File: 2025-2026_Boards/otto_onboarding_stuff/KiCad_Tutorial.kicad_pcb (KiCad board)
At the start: 2 copper layers, 28 parts, among them J1 USB_B_Micro, J2 Conn_01x04_Pin, J3 Conn_01x04_Pin, J4 Conn_01x04_Pin, SW1 SW_SPDT, U1 STM32F103C8T6, U3 AMS1117-3.3, Y1 16MHz

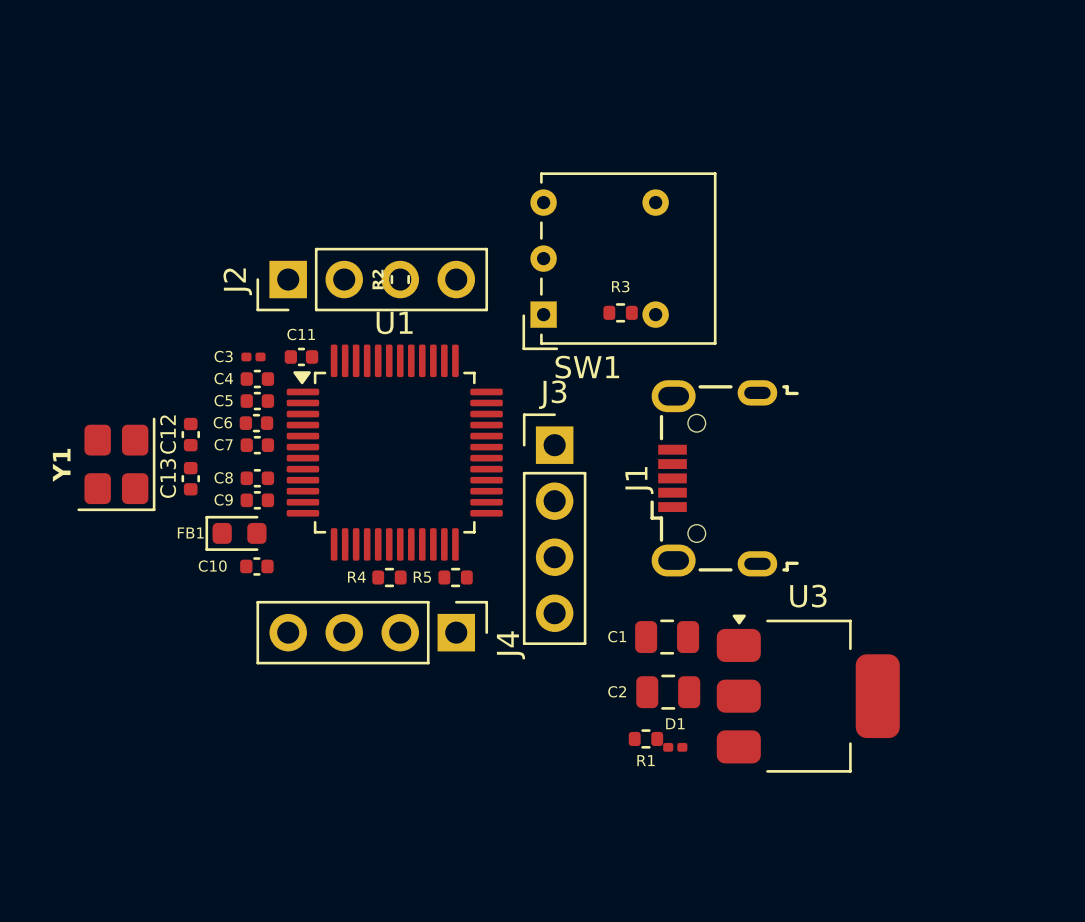
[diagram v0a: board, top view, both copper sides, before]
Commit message: Worked on wiring.
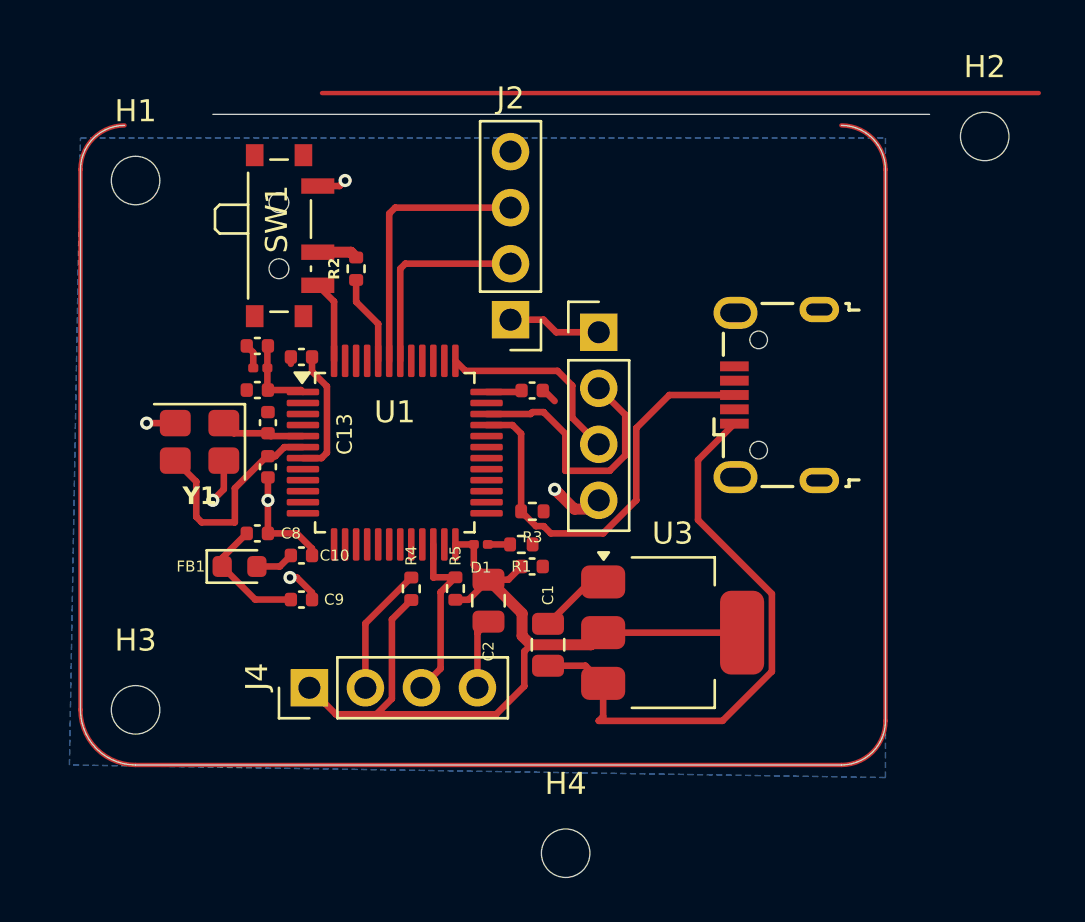
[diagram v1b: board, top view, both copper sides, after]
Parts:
- added H1: MountingHole, MountingHole:MountingHole_2.2mm_M2, F.Cu at (89.5, 64.0)
- added H2: MountingHole, MountingHole:MountingHole_2.2mm_M2, F.Cu at (128.0, 62.0)
- added H3: MountingHole, MountingHole:MountingHole_2.2mm_M2, F.Cu at (89.5, 88.0)
- added H4: MountingHole, MountingHole:MountingHole_2.2mm_M2, F.Cu at (109.0, 94.5)
- SW1: footprint Button_Switch_THT:SW_Lever_1P2T_NKK_GW12LxH -> Button_Switch_SMD:SW_SPDT_PCM12
- moved C7 13.6 mm to (107.5, 81.5), turned to 0 degrees
- moved D1 12.7 mm to (105.2, 80.5), turned to 180 degrees
- moved C5 12.5 mm to (107.5, 73.5)
- moved SW1 12.2 mm to (96.3, 66.5), turned to -90 degrees
- moved R1 10.5 mm to (107.0, 80.5)
- moved J2 10.2 mm to (106.5, 70.3), turned to 180 degrees
- moved R3 9.85 mm to (107.5, 79.0), turned to 180 degrees
- moved C2 9.15 mm to (105.5, 83.0), turned to -90 degrees
- moved J4 7.11 mm to (97.4, 87.0), turned to 90 degrees
- moved U3 6.79 mm to (113.8, 84.5)
- moved J3 5.50 mm to (110.5, 70.9)
- moved C1 5.41 mm to (108.2, 85.0), turned to 90 degrees
- moved C9 4.92 mm to (97.0, 83.0)
- moved J1 4.71 mm to (118.5, 73.7)
- moved Y1 3.91 mm to (92.4, 75.8), turned to 180 degrees
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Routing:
- net +3.3V: track 0.00 -> 54.5 mm
- net VBUS: track 0.00 -> 26.7 mm
- net GND: track 0.00 -> 22.8 mm, vias 0 -> 6
- net /USB_D+: track 0.00 -> 19.9 mm
- net /USART1_RX: track 0.00 -> 12.3 mm
- net /SDIO: track 0.00 -> 12.2 mm
- net /HSE_OUT: track 0.00 -> 10.2 mm
- net /USART1_TX: track 0.00 -> 9.27 mm
- net /SWCLK: track 0.00 -> 8.92 mm
- net /I2C2_STA: track 0.00 -> 8.34 mm
- net /I2C2_STL: track 0.00 -> 5.86 mm
- net /NRST: track 0.00 -> 5.81 mm
- net +3.3VA: track 0.00 -> 5.70 mm
- net /BOOT0: track 0.00 -> 4.08 mm
- net /HSE_IN: track 0.00 -> 3.83 mm
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- added copper zone on B.Cu, net GND
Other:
- board outline added: 38.5 x 29.5 mm
